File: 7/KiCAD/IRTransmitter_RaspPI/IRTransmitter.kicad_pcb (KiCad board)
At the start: 2 copper layers, 24.1 x 42.5 mm, 12 parts, among them J1 Conn_02x08_Odd_Even, Q1 BC33740TA, Q2 BC33740TA

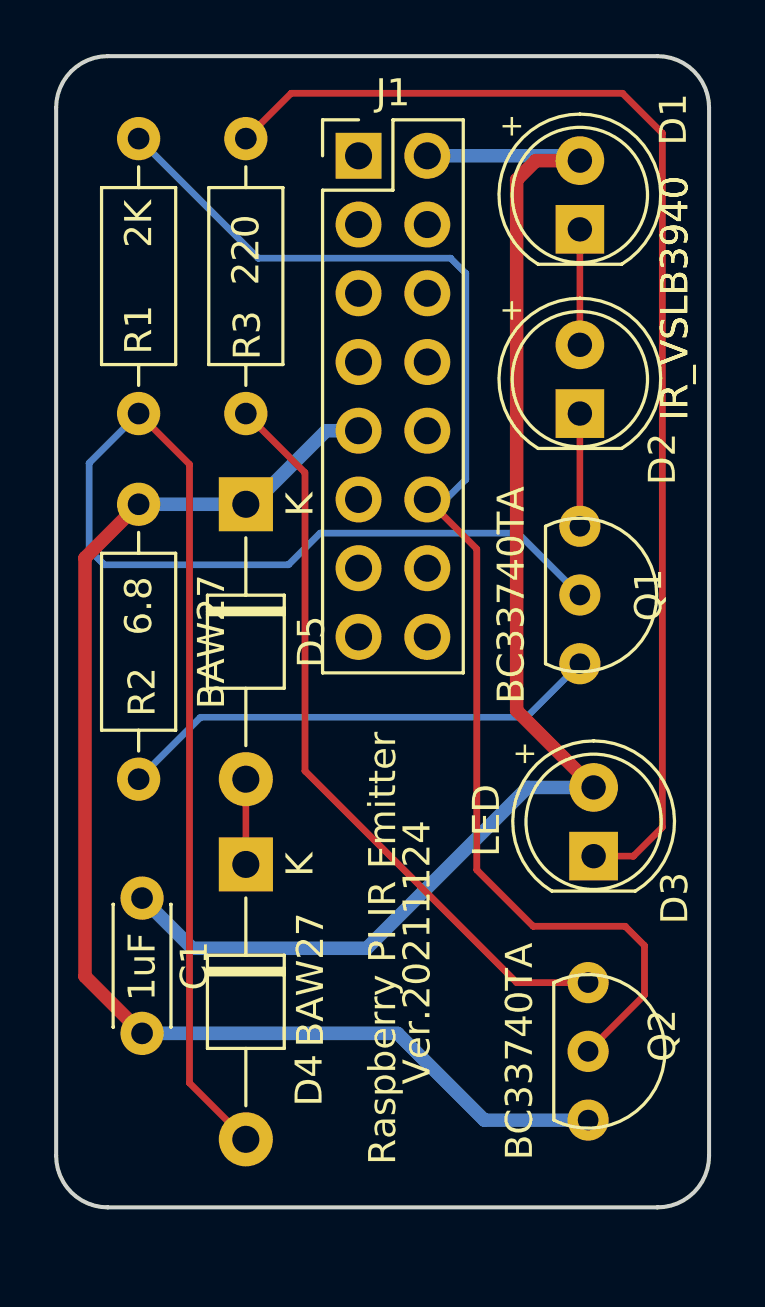
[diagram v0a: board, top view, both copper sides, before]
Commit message: Optimizing PCB
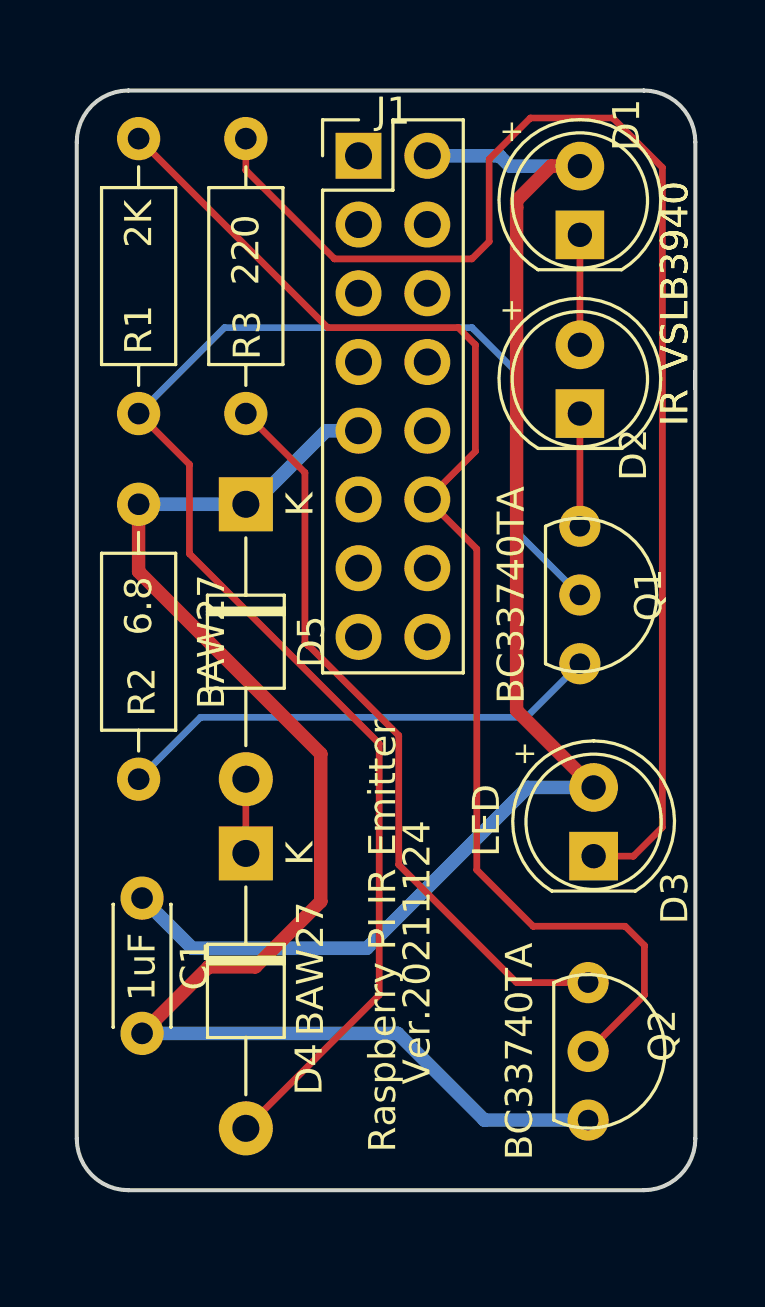
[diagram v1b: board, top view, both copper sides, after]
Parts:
- moved D4 0.41 mm to (64.2, 105.7)
- moved D1 0.20 mm to (76.5, 82.8)
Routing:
- net GND: track 48.3 -> 53.2 mm
- net Net-(D3-Pad1): track 45.3 -> 50.0 mm
- net Net-(D4-Pad2): track 54.0 -> 57.3 mm
- net /GPIO18: track 50.1 -> 48.6 mm
- net +5V: track 52.5 -> 51.4 mm
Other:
- board size 24.1 x 42.5 mm -> 22.9 x 40.6 mm
